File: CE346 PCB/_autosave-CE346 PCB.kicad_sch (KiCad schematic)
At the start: 56 parts, among them IC1 nRF52833-QDAA-R, J1 Conn_02x04_Odd_Even, J10 Conn_01x03_Pin, J2 Conn_01x02_Pin, J3 Conn_02x04_Odd_Even, J4 micro usb, J5 Conn_01x03_Pin, J6 micro usb, J7 Conn_01x03_Pin, J8 Conn_01x03_Pin, J9 Conn_01x03_Pin, SW1 SW_Push, SW2 SW_Push, U1 ESP32-WROOM-32E-N4, U2 SN74LV1T32DCKRG4, Y1 Crystal_GND23

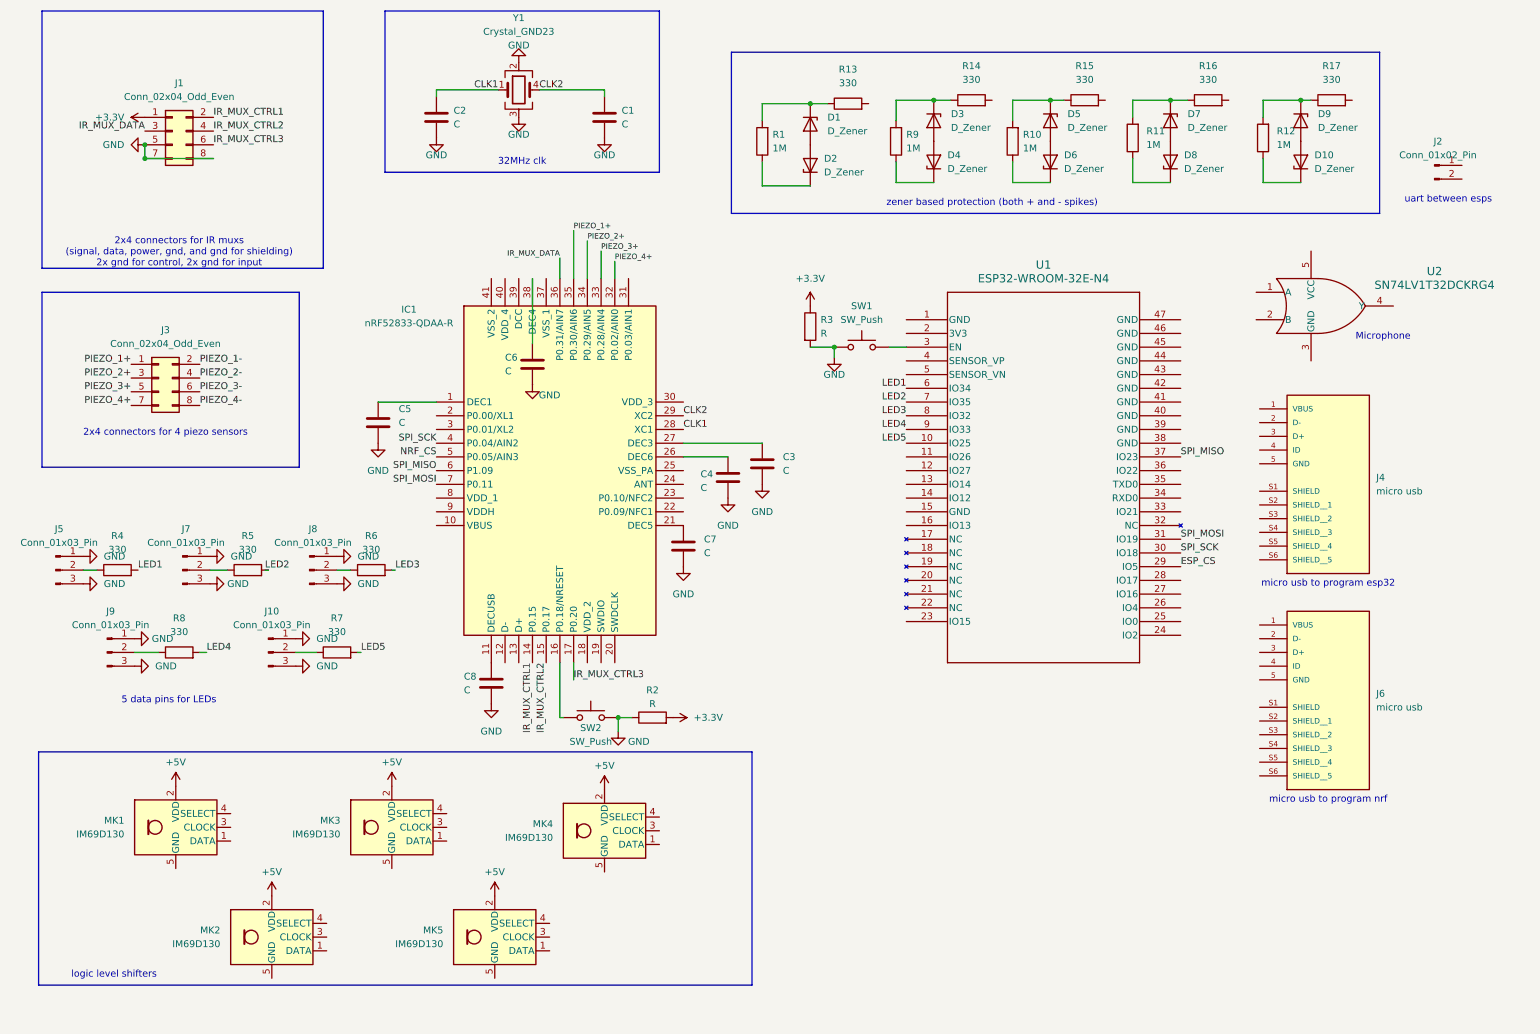
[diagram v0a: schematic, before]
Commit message: scjemaitc
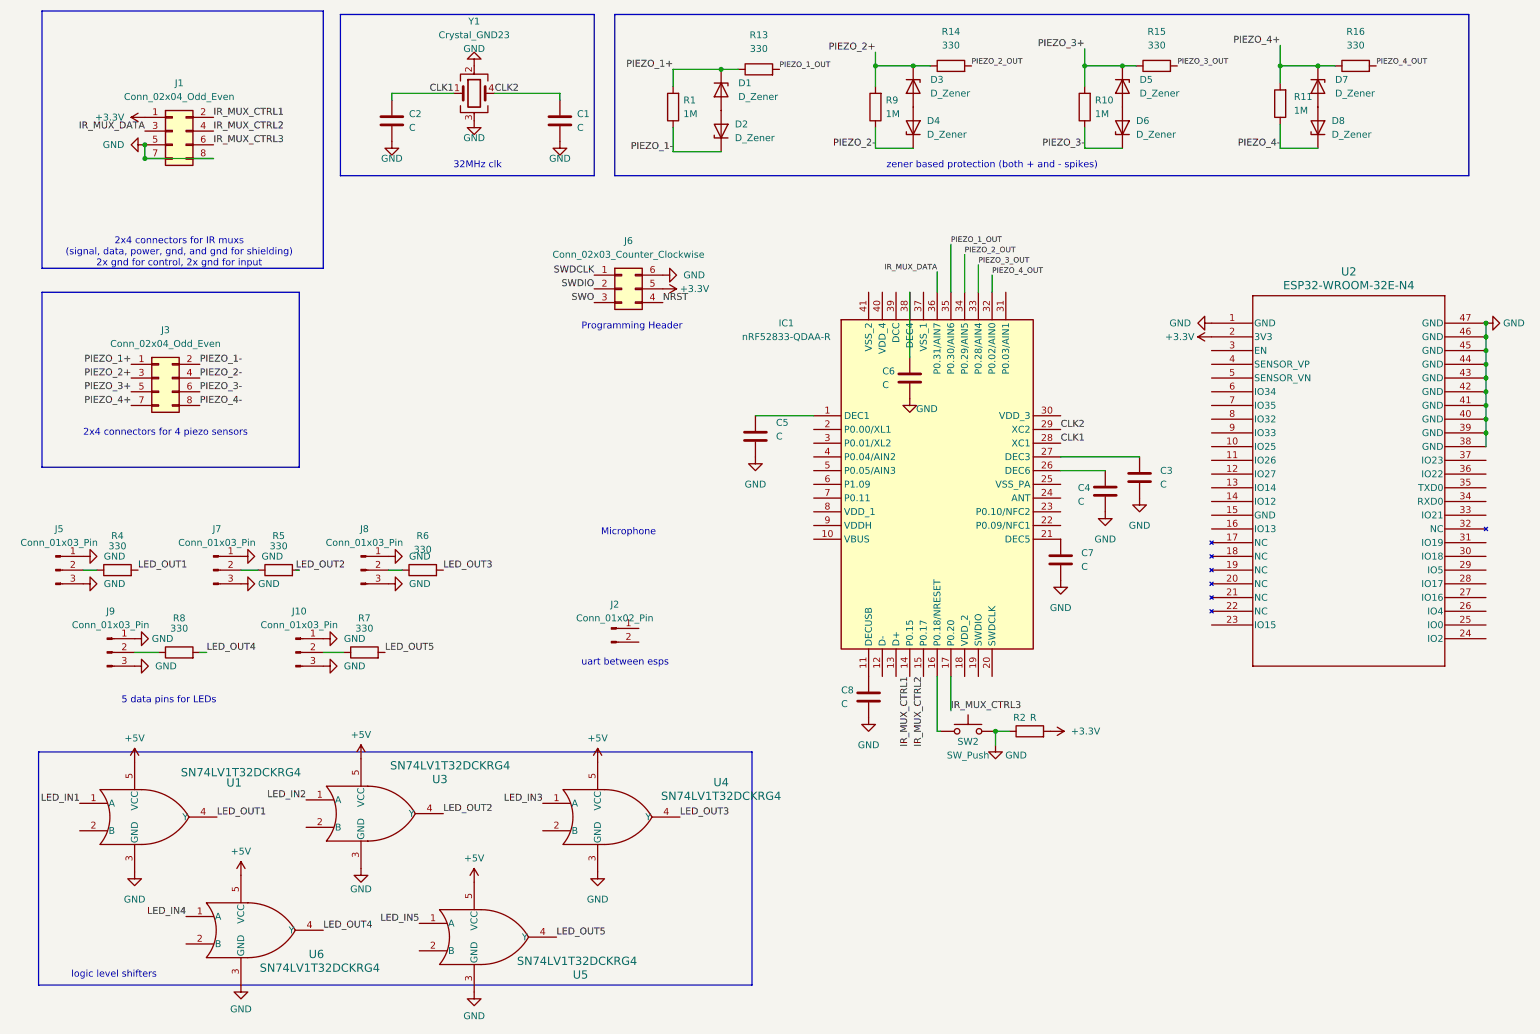
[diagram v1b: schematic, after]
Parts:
- removed D10, D9: D_Zener, symbol Device:D_Zener
- removed J4, J6: micro usb, 629105150921:WURTH_629105150921, symbol CE346 Symbols:micro usb
- removed MK1, MK2, MK3, MK4, MK5: IM69D130, CE346 Footprints:Logic_level_shifter, symbol Sensor_Audio:IM69D130
- removed R12: 1M, symbol Device:R
- removed R17: 330, symbol Device:R
- removed R3: R, symbol Device:R
- removed SW1: SW_Push, symbol Switch:SW_Push
- removed U1: ESP32-WROOM-32E-N4, symbol CE346 Symbols:ESP32-WROOM-32E-N4
- removed U2: SN74LV1T32DCKRG4, DCK0005A_N, symbol CE346 Symbols:SN74LV1T32DCKRG4
- added J6: Conn_02x03_Counter_Clockwise, symbol Connector_Generic:Conn_02x03_Counter_Clockwise
- added U1, U3, U4, U5, U6: SN74LV1T32DCKRG4, DCK0005A_N, symbol CE346 Symbols:SN74LV1T32DCKRG4
- added U2: ESP32-WROOM-32E-N4, symbol CE346 Symbols:ESP32-WROOM-32E-N4
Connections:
- net +3.3V: now also J6.5 (Pin_5), U2.2 (3V3)
- net +5V: now also U1.5 (VCC), U3.5 (VCC), U4.5 (VCC), U5.5 (VCC), U6.5 (VCC)
- net GND: now also J6.6 (Pin_6), U1.3 (GND), U2.1 (GND), U2.38 (GND), U2.39 (GND), U2.40 (GND), U2.41 (GND), U2.42 (GND), U2.43 (GND), U2.44 (GND), U2.45 (GND), U2.46 (GND), U2.47 (GND), U3.3 (GND), U4.3 (GND), U5.3 (GND), U6.3 (GND)
- net PIEZO_1+: now also D1.1 (K), R1.2, R13.1; no longer IC1.35 (P0.30/AIN6)
- net PIEZO_1-: now also D2.1 (K), R1.1
- net PIEZO_2+: now also D3.1 (K), R14.1, R9.2; no longer IC1.34 (P0.29/AIN5)
- net PIEZO_2-: now also D4.1 (K), R9.1
- net PIEZO_3+: now also D5.1 (K), R10.2, R15.1; no longer IC1.33 (P0.28/AIN4)
- net PIEZO_3-: now also D6.1 (K), R10.1
- net PIEZO_4+: now also D7.1 (K), R11.2, R16.1; no longer IC1.32 (P0.02/AIN0)
- net PIEZO_4-: now also D8.1 (K), R11.1
- net PIEZO_2_OUT: now reaches R14.2
- net PIEZO_2_OUT: now also IC1.34 (P0.29/AIN5)
- net PIEZO_4_OUT: now reaches R16.2
- net PIEZO_4_OUT: now also IC1.32 (P0.02/AIN0)
- net PIEZO_3_OUT: now reaches R15.2
- net PIEZO_3_OUT: now also IC1.33 (P0.28/AIN4)
- net PIEZO_1_OUT: now reaches R13.2
- net PIEZO_1_OUT: now also IC1.35 (P0.30/AIN6)
- net LED1 renamed LED_OUT1
- net LED_OUT1: now also U1.4 (Y)
- net LED2 renamed LED_OUT2
- net LED_OUT2: now also U3.4 (Y)
- net LED3 renamed LED_OUT3
- net LED_OUT3: now also U4.4 (Y)
- net LED4 renamed LED_OUT4
- net LED_OUT4: now also U6.4 (Y)
- net LED5 renamed LED_OUT5
- net LED_OUT5: now also U5.4 (Y)
- net NRF_CS: no longer names the net of IC1.5 (P0.05/AIN3)
- net SPI_MISO: no longer names the net of IC1.6 (P1.09)
- net SPI_MOSI: no longer names the net of IC1.7 (P0.11)
- net SPI_SCK: no longer names the net of IC1.4 (P0.04/AIN2)
- new net LED_IN1: U1.1 (A)
- new net LED_IN2: U3.1 (A)
- new net LED_IN3: U4.1 (A)
- new net LED_IN4: U6.1 (A)
- new net LED_IN5: U5.1 (A)
- new net NRST: J6.4 (Pin_4)
- new net SWDCLK: J6.1 (Pin_1)
- new net SWDIO: J6.2 (Pin_2)
- new net SWO: J6.3 (Pin_3)
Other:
- note added: "Programming Header"
- note removed: "micro usb to program esp32"
- note removed: "micro usb to program nrf"
- moved on the sheet: C1, C2, C3, C4, C5, C6, C7, C8, D1, D2, D3, D4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
